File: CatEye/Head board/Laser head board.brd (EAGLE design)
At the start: 70.3 x 28.4 mm, 18 parts, among them X1 DVI-D-R, X2 SMA-R

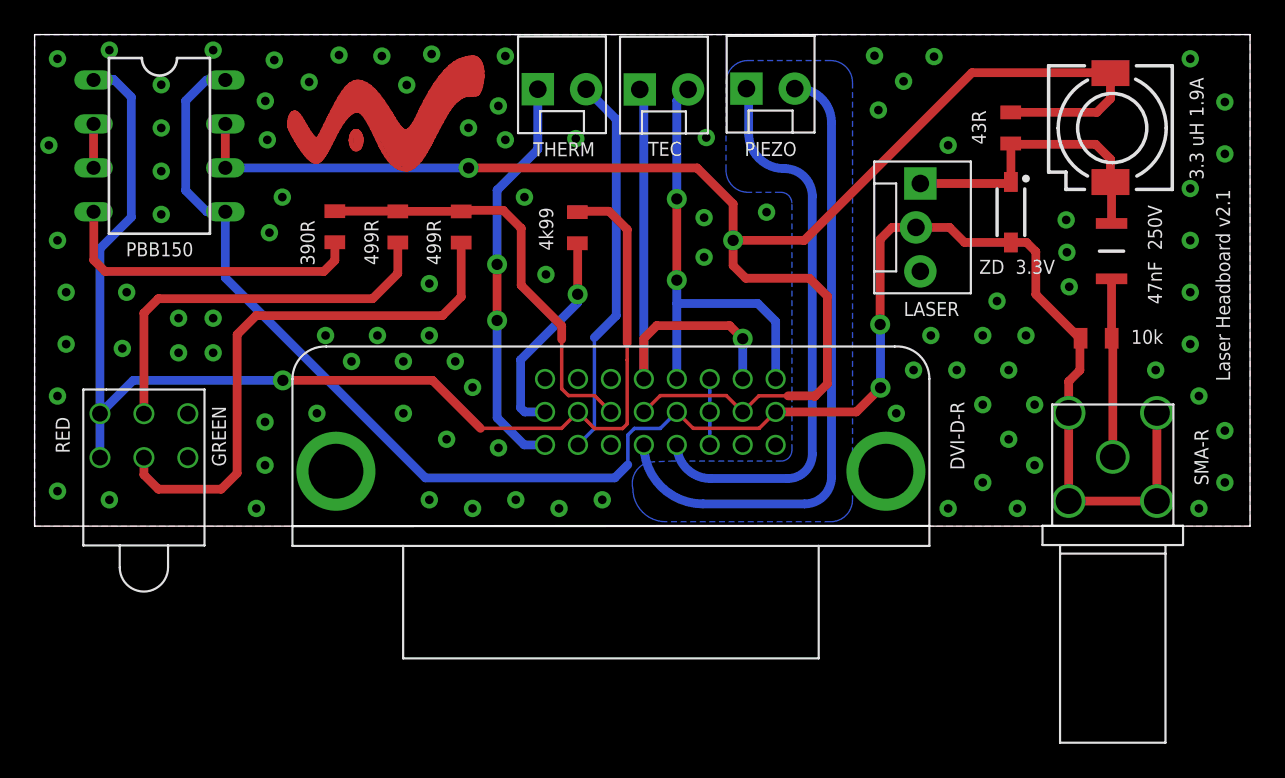
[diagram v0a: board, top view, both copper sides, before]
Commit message: STEP files
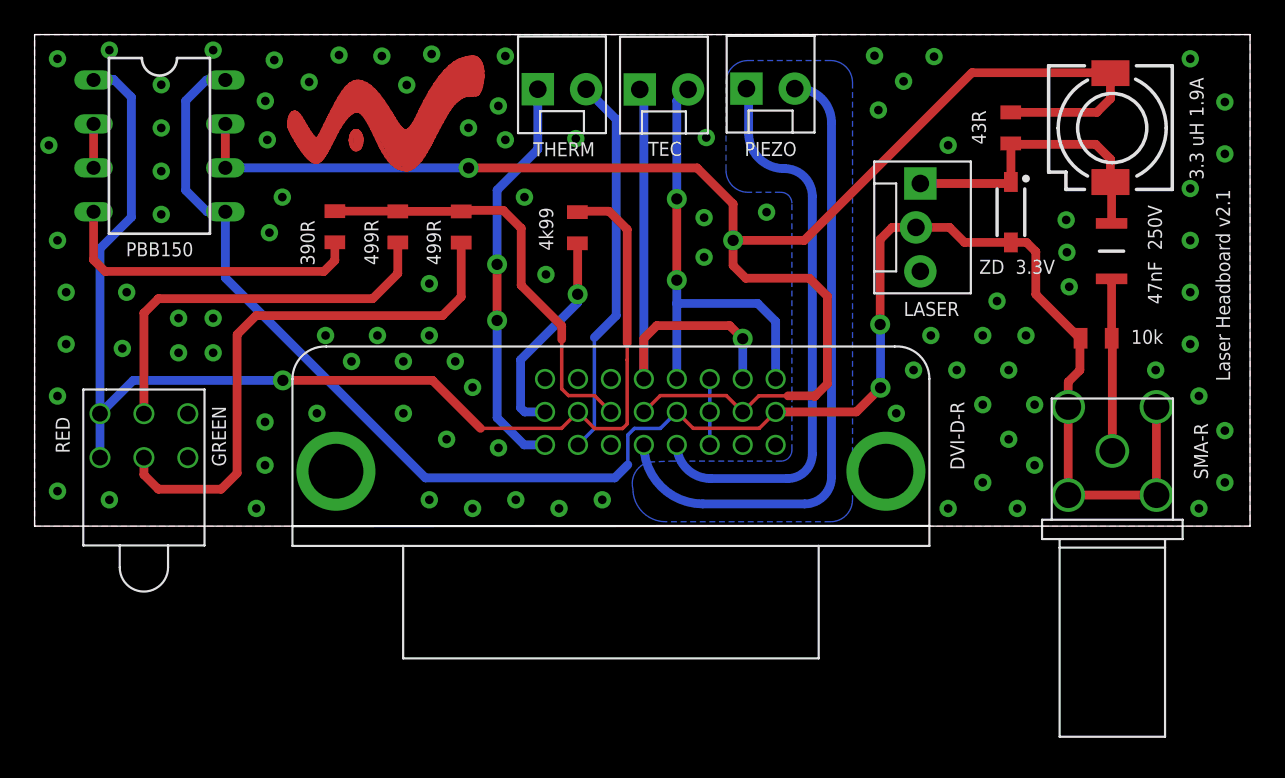
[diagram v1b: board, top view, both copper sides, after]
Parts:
- C1: device OCR:CAPC3216X180N -> headboard:OCR_CAPC3216X180N
- L1: device OCR:INDC7070 -> headboard:OCR_INDC7070
- LASER: device OCR:MOLEX-1X3_LOCK -> headboard:OCR_MOLEX-1X3_LOCK
- LD1: device OCR:WP130WCP/2EGW -> headboard:OCR_WP130WCP/2EGW
- PBB150: device OCR:DIL08 -> headboard:OCR_DIL08
- PIEZO, TEC, THERM: device OCR:MOLEX-1X2_LOCK -> headboard:OCR_MOLEX-1X2_LOCK
- R1, R2, R3, R4, R5, R6: device OCR:0805 -> headboard:OCR_0805
- X1: device OCR:DVI-D-R -> headboard:OCR_DVI-D-R
- X2: device OCR:SMA_0732512201 -> headboard:OCR_SMA_0732512201
- ZD: device OCR:SOD3716X135N -> headboard:OCR_SOD3716X135N
- moved X2 0.35 mm to (29.0, 2.82)
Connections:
- net N$7: now also PBB150.4; no longer PBB150.3
- net N$8: now also PBB150.3; no longer PBB150.4
